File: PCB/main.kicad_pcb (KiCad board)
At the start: 2 copper layers, 90 x 90 mm, 37 parts, among them J1 ATX-24, J10 Conn_USB_HUBS, J11 Conn_USB_HUBS, J12 POWER_ON, J2 Conn_RPi, J3 Conn_USB_HUBS, J4 Conn_Router, J5 Conn_MOBILE, J6 Conn_NUC, J7 Conn_USB_HUBS, J8 Conn_USB_HUBS, J9 Conn_USB_HUBS

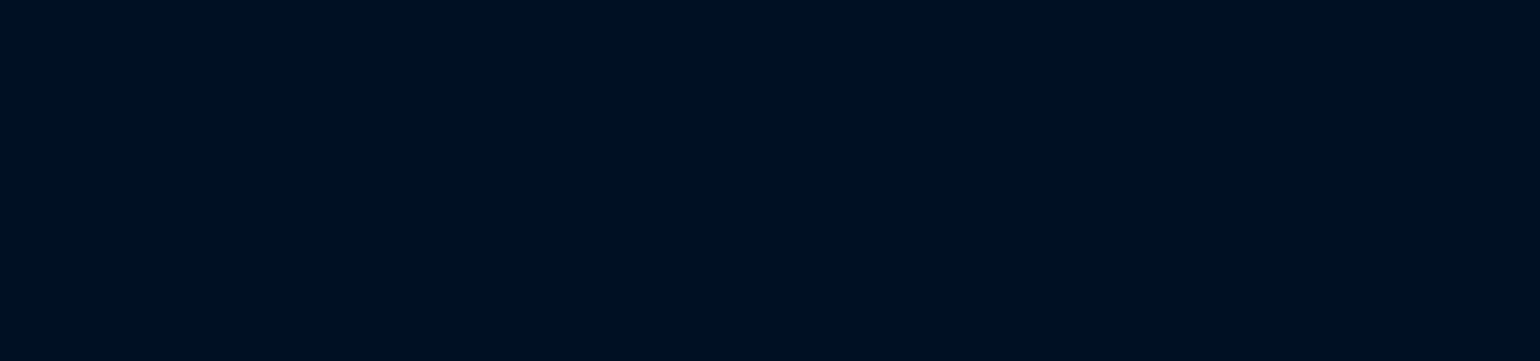
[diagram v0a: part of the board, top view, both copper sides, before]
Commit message: update mobile-test-stand-tryout,
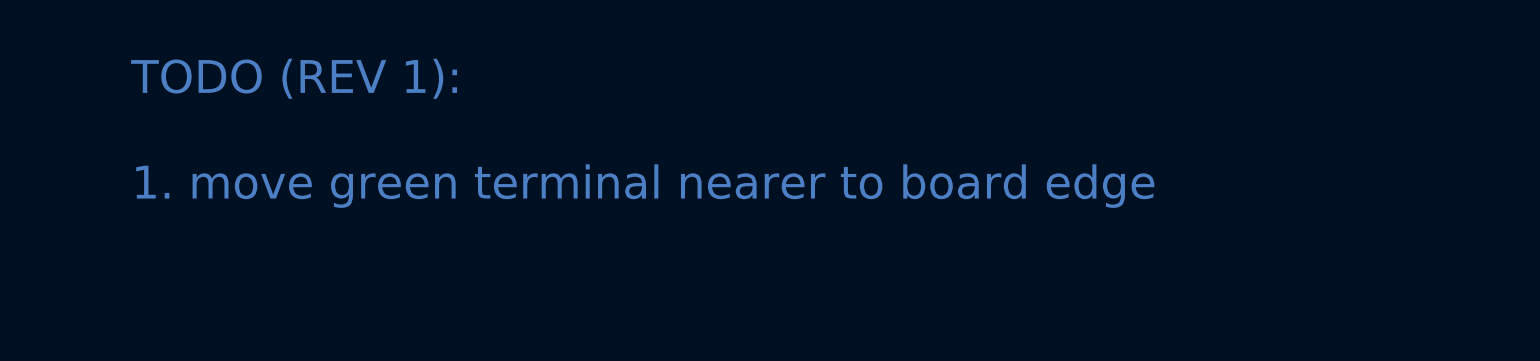
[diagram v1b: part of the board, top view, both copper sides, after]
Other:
- board text added: "TODO (REV 1): 1. move green terminal nearer to board edge"
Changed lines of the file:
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@@
+    (effects (font (size 1.5 1.5) (thickness 0.3)) (justify left))
+  )
+  (gr_text "TODO (REV 1):\n\n1. move green terminal nearer to board edge" (at 194 25) (layer "B.Cu")
     (effects (font (size 1.5 1.5) (thickness 0.3)) (justify left))
   )

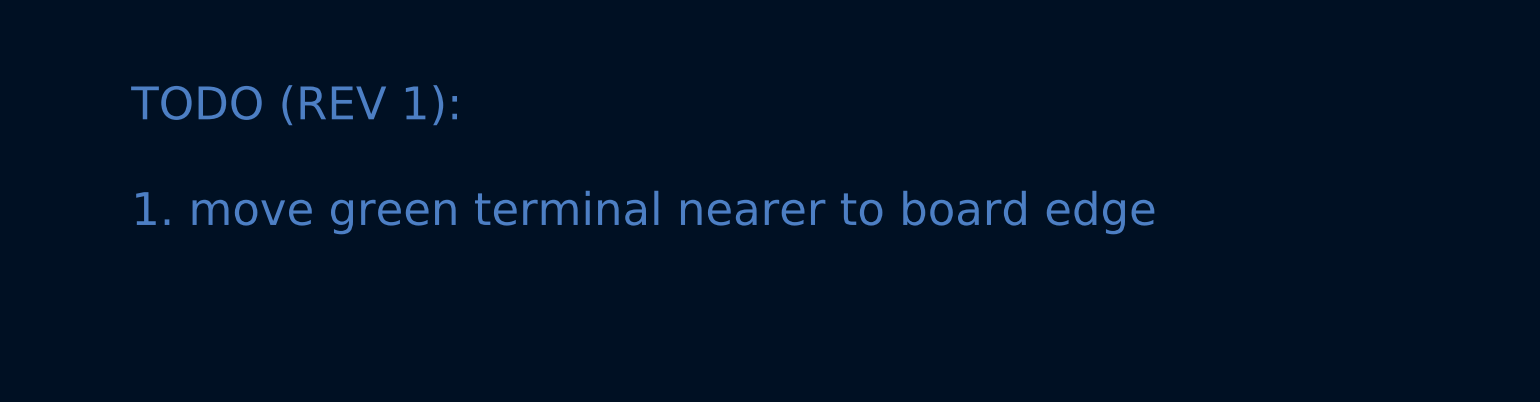
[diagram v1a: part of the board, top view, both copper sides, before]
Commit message: update mobile-test-stand-tryout,
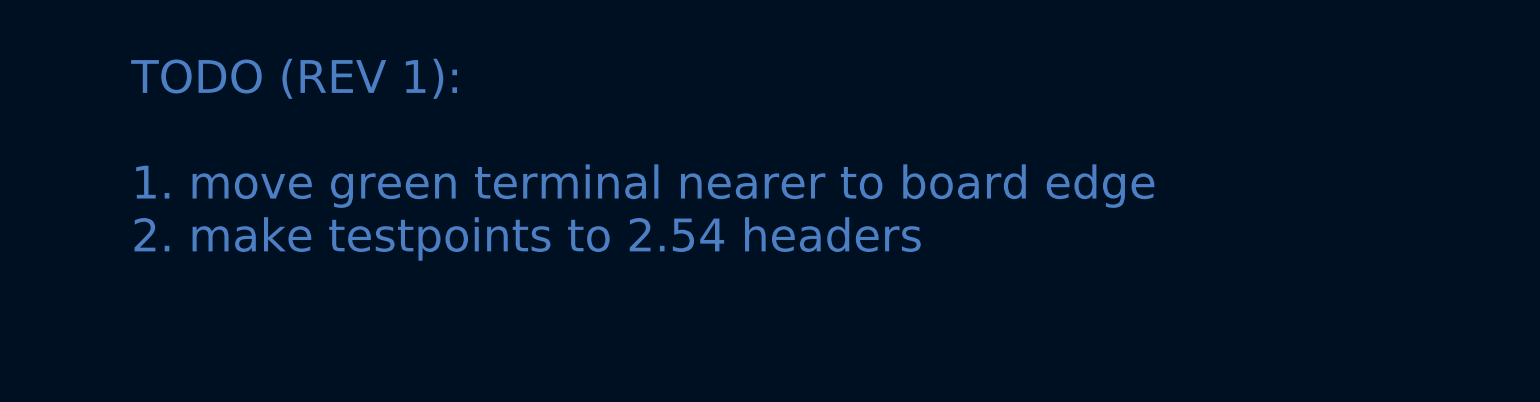
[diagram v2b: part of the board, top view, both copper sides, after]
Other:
- board text added: "TODO (REV 1): 1. move green terminal nearer to board edge 2. make testpoints to 2.54 headers"
- board text removed: "TODO (REV 1): 1. move green terminal nearer to board edge"
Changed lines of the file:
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@@
     (effects (font (size 1.5 1.5) (thickness 0.3)) (justify left))
   )
-  (gr_text "TODO (REV 1):\n\n1. move green terminal nearer to board edge" (at 194 25) (layer "B.Cu")
+  (gr_text "TODO (REV 1):\n\n1. move green terminal nearer to board edge\n2. make testpoints to 2.54 headers" (at 194 25) (layer "B.Cu")
     (effects (font (size 1.5 1.5) (thickness 0.3)) (justify left))
   )
